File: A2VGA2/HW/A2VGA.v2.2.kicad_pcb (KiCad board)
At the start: 2 copper layers, 65.5 x 79.8 mm, 66 parts, among them U1 CPB

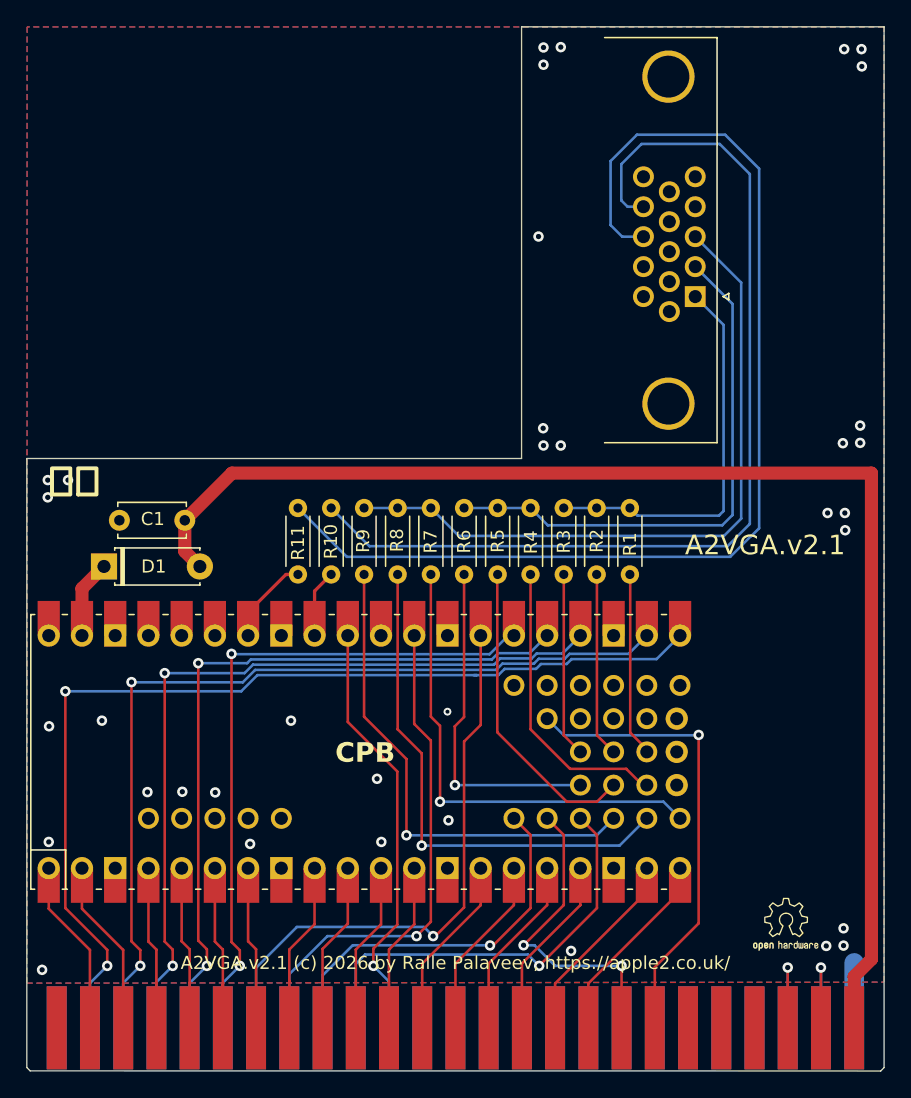
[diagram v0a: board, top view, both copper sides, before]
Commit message: Add files via upload
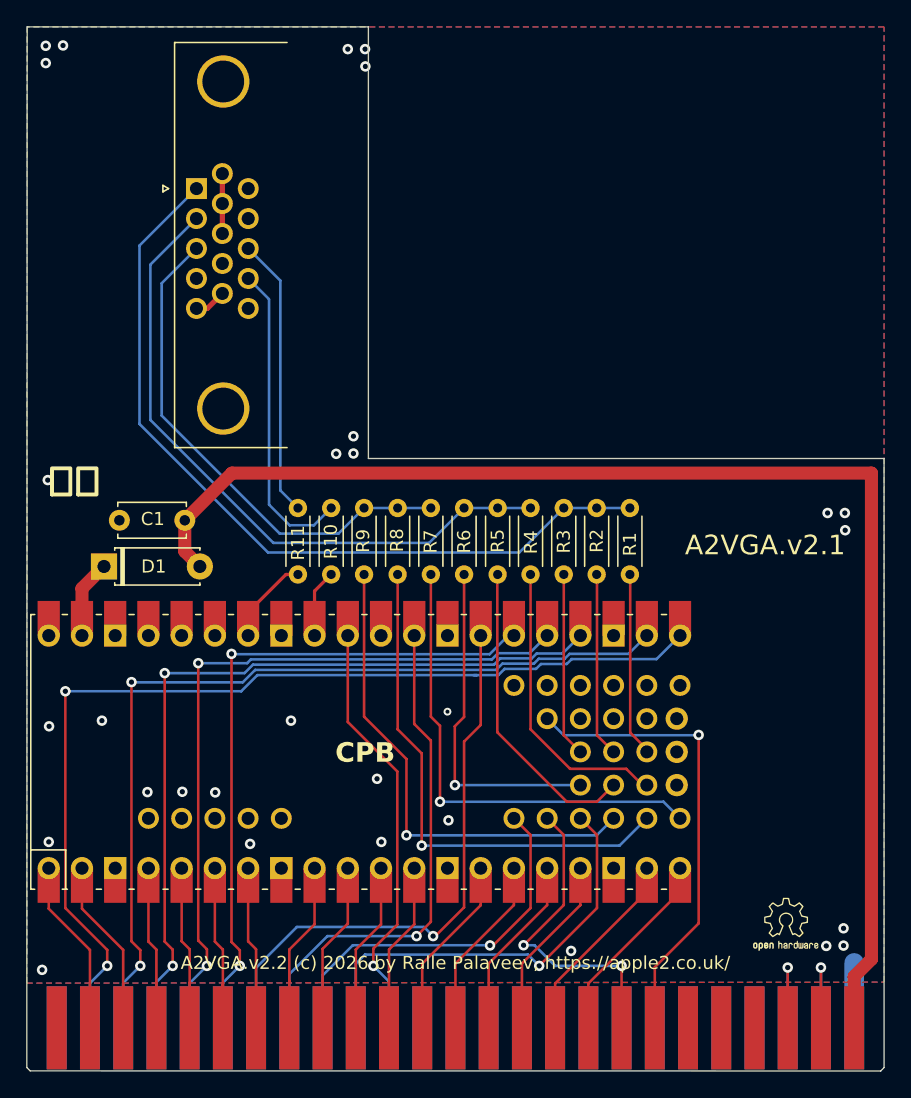
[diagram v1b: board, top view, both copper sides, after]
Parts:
- moved H3 39.0 mm to (125.0, 71.4), turned to 90 degrees
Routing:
- net HS_out: track 86.2 -> 21.4 mm
- net VS_out: track 76.7 -> 23.9 mm
- net R_out: track 29.9 -> 62.8 mm
- net B_out: track 52.5 -> 38.3 mm
- net G_out: track 41.6 -> 50.9 mm
- net GND: track 4.95 -> 12.0 mm, vias 36 -> 30
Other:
- outline, holes or cut-outs redrawn
- board text added: "A2VGA.v2.2 (c) 2026 by Ralle Palaveev, https://apple2.co.uk/"
- board text removed: "A2VGA.v2.1 (c) 2026 by Ralle Palaveev, https://apple2.co.uk/"
